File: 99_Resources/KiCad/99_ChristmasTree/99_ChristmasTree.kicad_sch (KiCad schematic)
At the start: 9 parts, among them M1 SEN0539_VoiceCommand

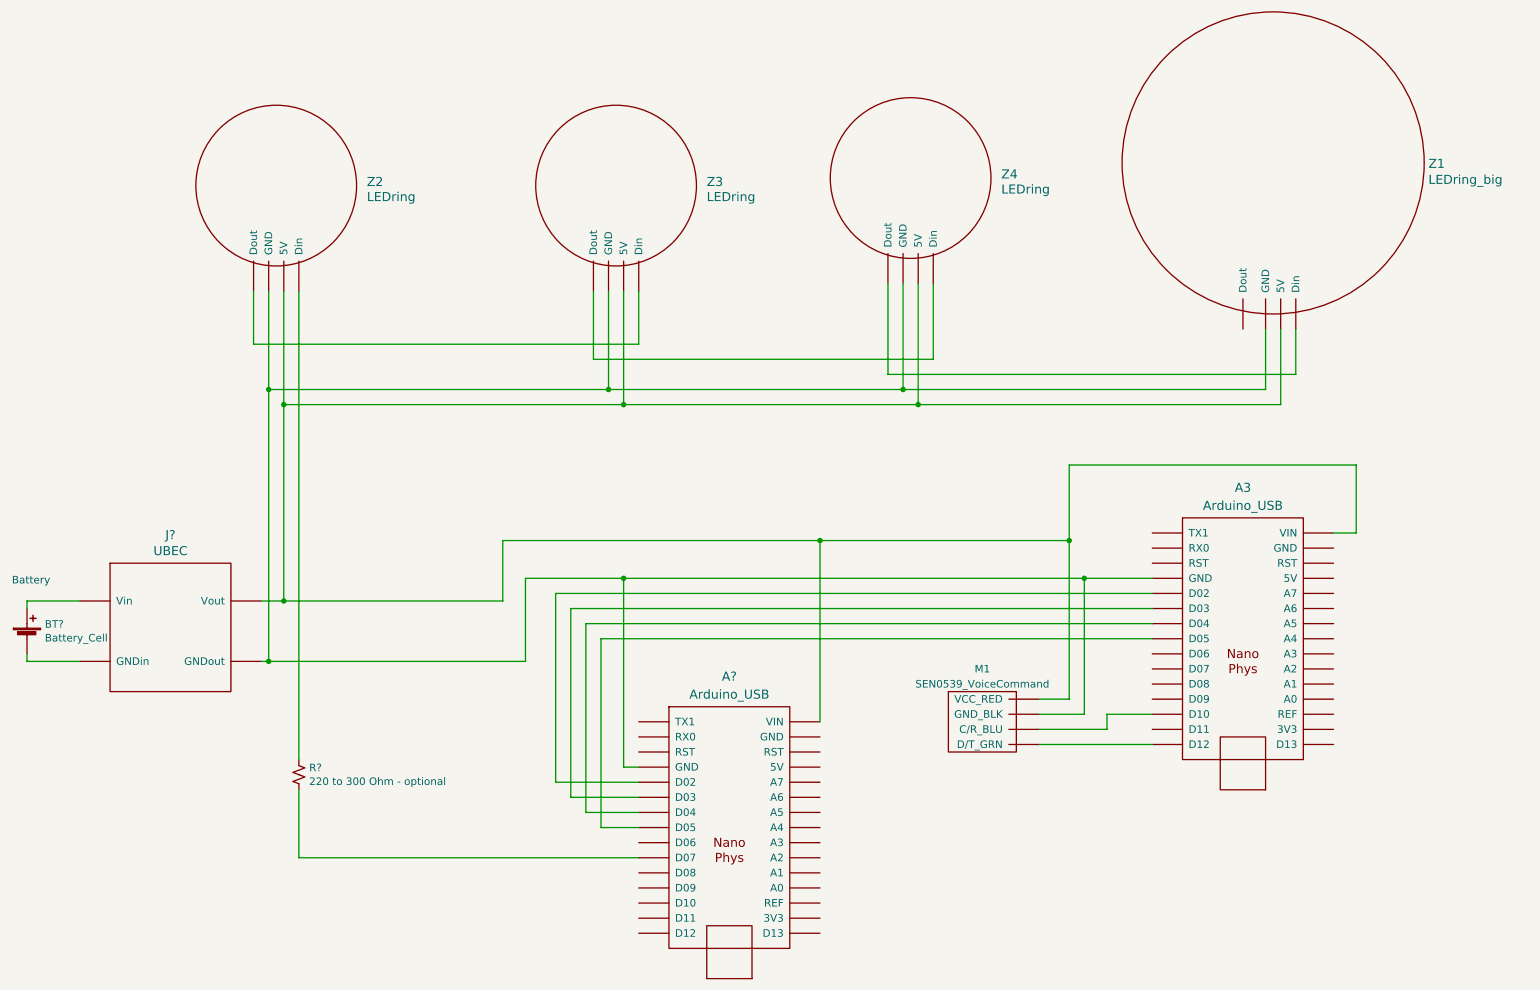
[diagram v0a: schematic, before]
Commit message: KiCad - make it neater
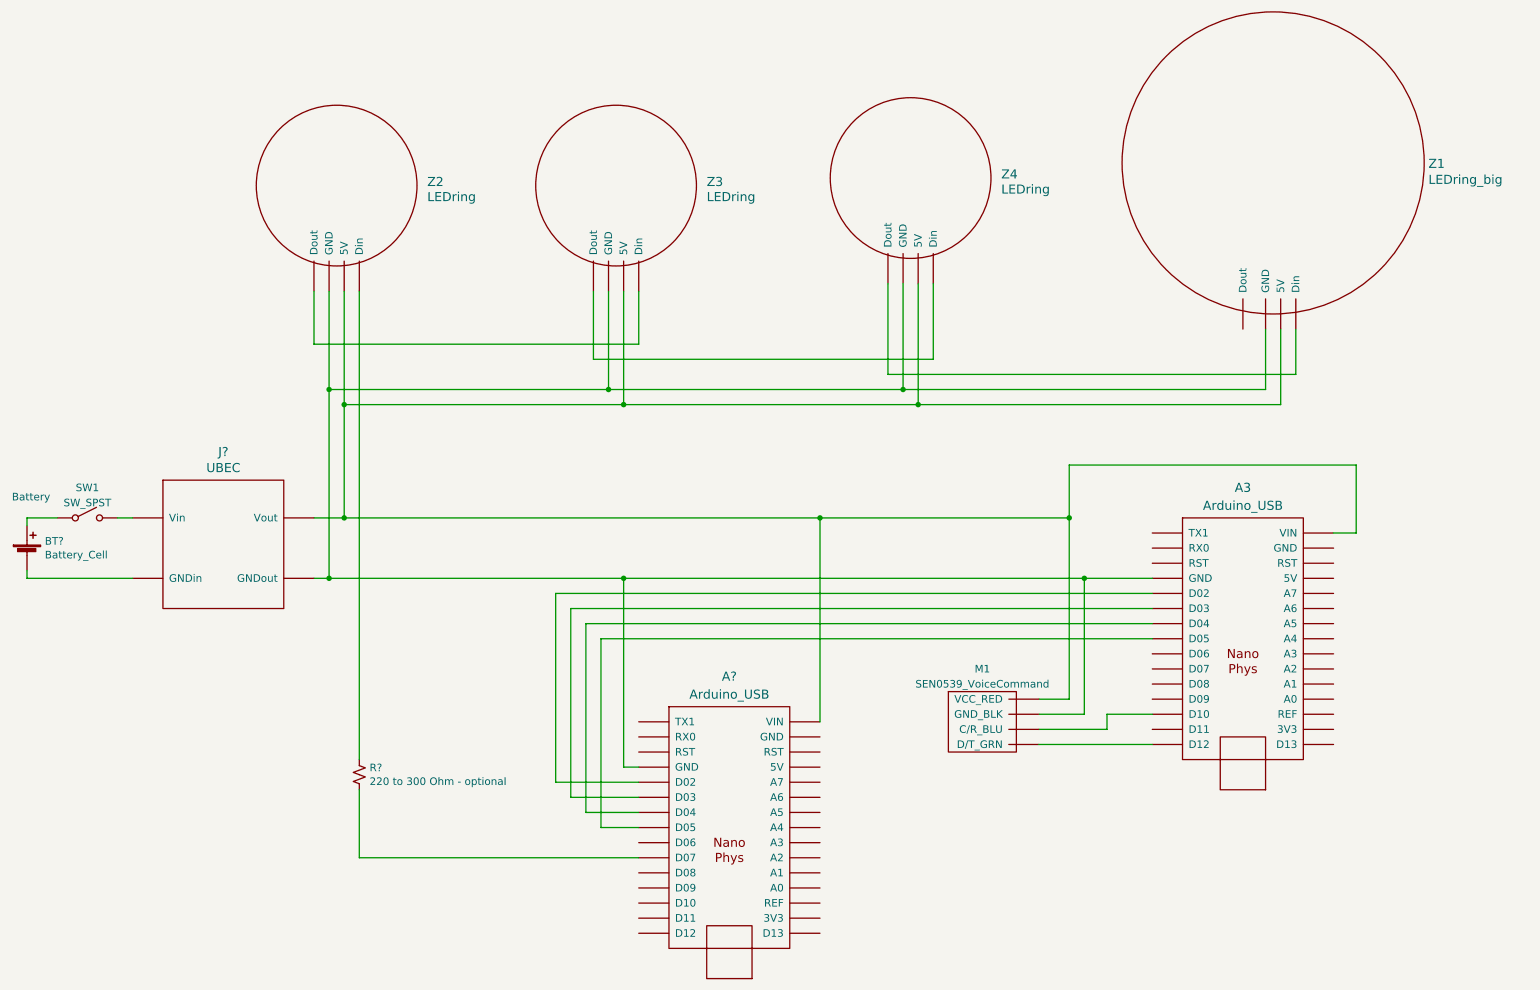
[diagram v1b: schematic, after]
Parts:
- added SW1: SW_SPST, symbol MDO:SW_SPST
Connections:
- net at A?.~ (VIN): now also A3.~ (VIN)
- net at A3.~ (VIN): no longer A?.~ (VIN)
- net at BT?.1 (+): now also SW1.~ (B)
- net at Z4.~ (GND): now also Z3.~ (GND); no longer Z1.~ (GND)
- net at Z3.~ (GND): now also Z2.~ (GND); no longer Z4.~ (GND)
- new net: A3.~ (VIN), A?.~ (VIN), M1.~ (VCC_RED), Z1.~ (GND), Z2.~ (GND), Z3.~ (GND), Z4.~ (GND) (x2)
- new net: A3.~ (VIN), A?.~ (VIN) (x3)
- new net: Z1.~ (GND), Z4.~ (GND)
- new net: A3.~ (VIN), M1.~ (VCC_RED)
- now unconnected: A3.~ (VIN), A3.~ (VIN), A3.~ (VIN), A3.~ (VIN), A3.~ (VIN), A3.~ (VIN), Z1.~ (GND), Z1.~ (GND)
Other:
- moved on the sheet: BT?, R?, Z2
